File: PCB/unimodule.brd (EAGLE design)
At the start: 103 x 74.2 mm, 150 parts, among them IC1 TTGO_DISP, IC2 DS18D20, IC3 FAN3111E, IC4 FAN3111E, IC5 FAN3111E, K1 XY2500(5.0)-4PV, K100 G5LE-1-E 5VDC OMRON, K101 XY2500(5.0)-4PV, K102 JST-B02B-JWPF-SK-R, K103 JST-B04B-JWPF-SK-R, K104 JST-B08B-JWPF-SK-R, K105 JST-B03B-JWPF-SK-R, U1 MAX3485, U2 LMR62014XMFE/NOPB0

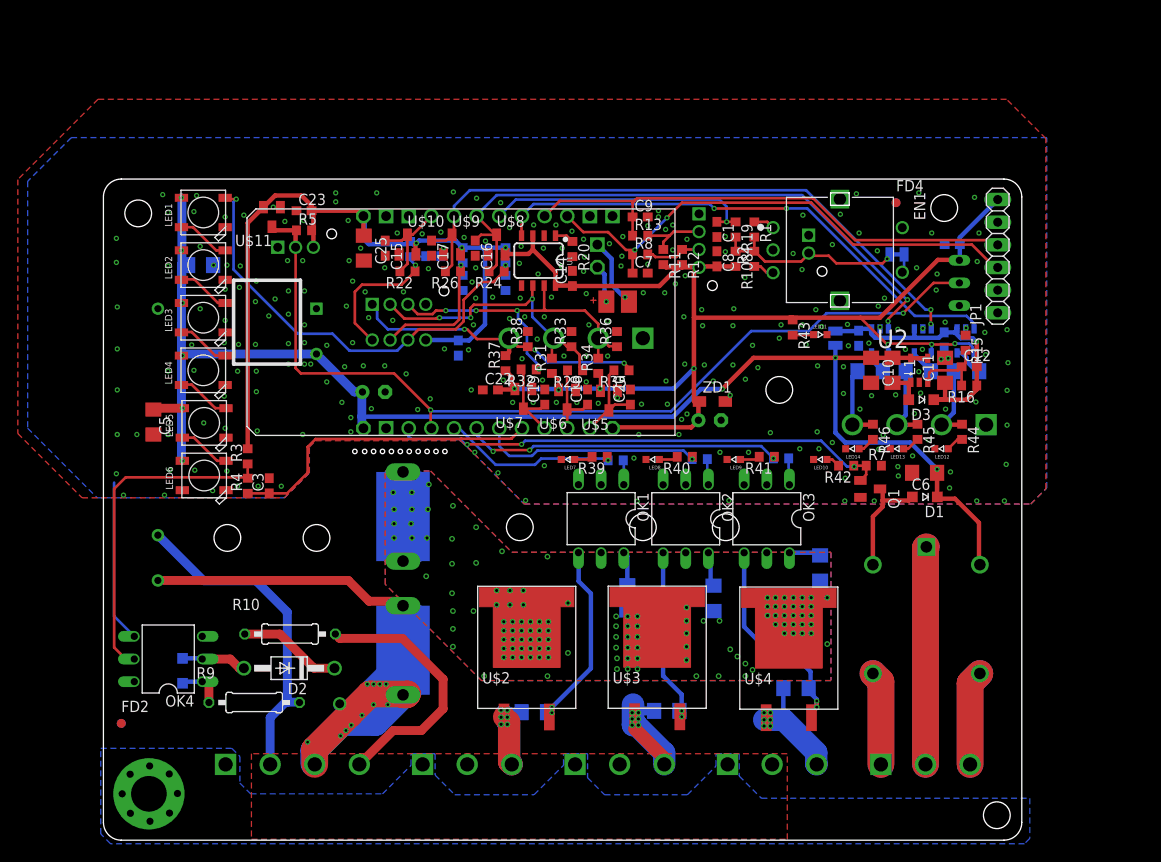
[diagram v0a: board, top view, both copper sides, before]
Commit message: silk screen organize
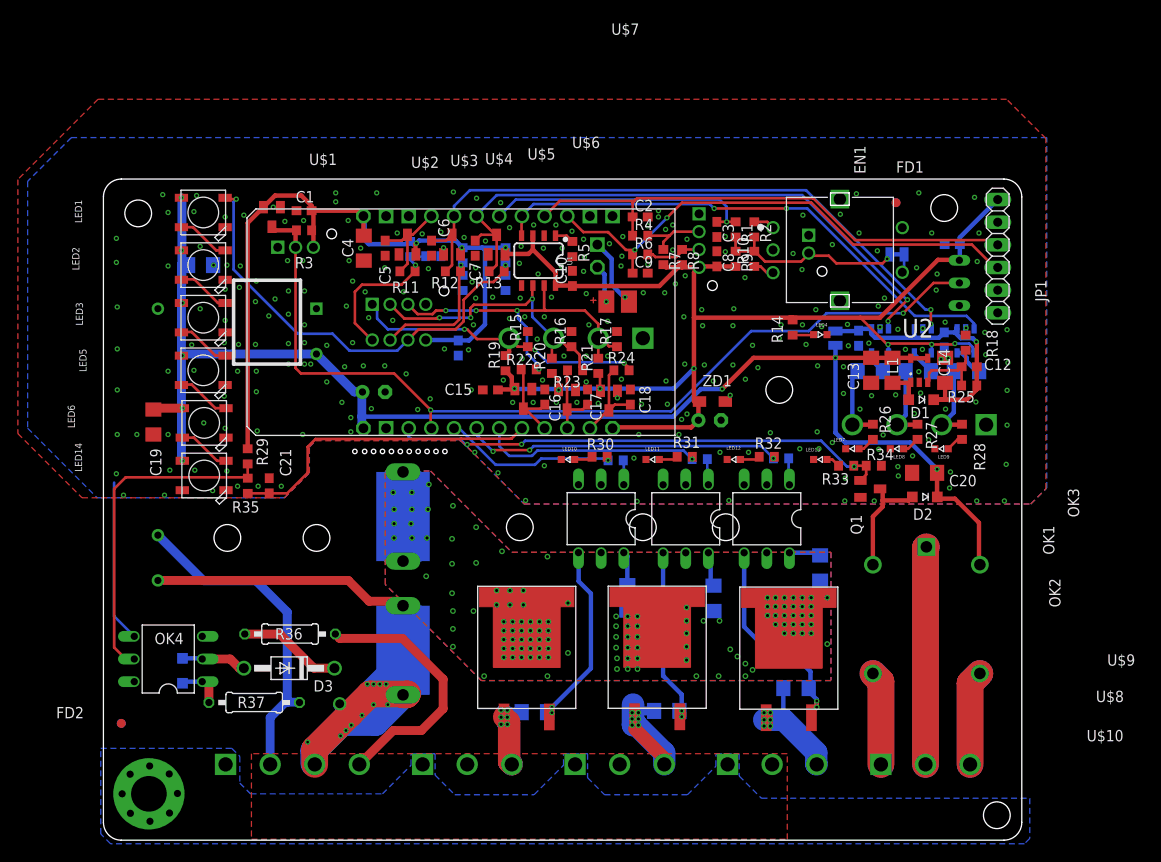
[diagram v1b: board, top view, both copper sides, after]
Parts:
- removed C22, C23: 100n, rcl:C0603
- removed C25: 22uF, rcl:C1206
- removed C26: DISP_BATSMD, TTGO_LCD_DISP:BAT_SMD
- removed FD3, FD4: (no value), siliXcon-pads:1-2MM-FIDUCIAL
- removed K1: XY2500(5.0)-4PV, siliXcon-connectors:XY2500V-B_4P
- removed R38: 10k, rcl:R0603
- removed R39, R40, R41, R42, R43: 220R, rcl:R0603
- removed R44, R45, R46: 1k, rcl:R0603
- removed SJ1: (no value), siliXcon-pads:SMD-JUMPER
- removed U$11: BAT54SFILM, siliXcon-semiconductors:PG-SOT23
- added C102, C103, C106: 100n, rcl:C0603
- added C105: 22uF, rcl:C1206
- added FD100, FD101: (no value), siliXcon-pads:1-2MM-FIDUCIAL
- added K106: JST-B03B-JWPF-SK-R, siliXcon-connectors:JST-B03B-JWPF-SK-R
- added R109, R110, R111: 1k, rcl:R1206
- added R112, R113, R114, R115, R116, R117: 10k, rcl:R0603
- added SJ101: (no value), siliXcon-pads:SMD-JUMPER-TIE
- added U$105: IRM-03-05, siliXcon-modules:IRM-03
- C1: value (none) -> 100n
- C10, C5, C6: value 22uF -> 100n; device rcl:C1206 -> rcl:C0603
- C11: value 22uF -> DISP_BATSMD; device rcl:C1206 -> TTGO_LCD_DISP:BAT_SMD
- C13, C14, C19, C20, C4: value 100n -> 22uF; device rcl:C0603 -> rcl:C1206
- C2: value 22uF -> !DNP 100n; device rcl:C1206 -> rcl:C0603
- C3: value 100n -> (none)
- C7: value !DNP 100n -> 100n
- D1: value (none) -> PMEG4005AEA
- D2: value 1N4004 -> (none); device diode:DO41-10 -> siliXcon-semiconductors:SOD123F
- D3: value PMEG4005AEA -> 1N4004; device siliXcon-semiconductors:SOD123F -> diode:DO41-10
- K102: value JST-B02B-JWPF-SK-R -> XY2500(5.0)-4PV; device siliXcon-connectors:JST-B02B-JWPF-SK-R -> siliXcon-connectors:XY2500V-B_4P
- K103: value JST-B04B-JWPF-SK-R -> JST-B08B-JWPF-SK-R; device siliXcon-connectors:JST-B04B-JWPF-SK-R -> siliXcon-connectors:JST-B08B-JWPF-SK-R
- K104: value JST-B08B-JWPF-SK-R -> JST-B04B-JWPF-SK-R; device siliXcon-connectors:JST-B08B-JWPF-SK-R -> siliXcon-connectors:JST-B04B-JWPF-SK-R
- K105: value JST-B03B-JWPF-SK-R -> JST-B02B-JWPF-SK-R; device siliXcon-connectors:JST-B03B-JWPF-SK-R -> siliXcon-connectors:JST-B02B-JWPF-SK-R
- LED14: value (none) -> WS2812B5050; device siliXcon-semiconductors:LED-0603 -> adafruit:WS2812B
- LED4: value WS2812B5050 -> (none); device adafruit:WS2812B -> siliXcon-semiconductors:LED-0603
- R10, R9: value 30k -> (none); device rcl:0207/10 -> rcl:R0603
- R105: value 220R -> 380R; device rcl:R0603 -> rcl:R1206
- R108: value (none) -> 220R
- R11, R12, R5: value 4k7 -> 100R
- R14: value 1k -> 220R; device rcl:R1206 -> rcl:R0603
- R15: value 6k8 -> 10k
- R16: value 47k -> 10k
- R17: value 1k -> 10k; device rcl:R1206 -> rcl:R0603
- R18: value 1k -> 6k8; device rcl:R1206 -> rcl:R0603
- R19: value (none) -> 10k
- R20: value 100R -> 10k
- R23: value 10k -> 100R
- R25: value 10k -> 47k
- R26, R29: value 100R -> 1k
- R27, R28: value 10k -> 1k
- R3: value 1k -> 4k7
- R30, R31, R33: value 10k -> 220R
- R32: value 100R -> 220R
- R34: value 10k -> 100k
- R35: value 100R -> 100k
- R36, R37: value 10k -> 30k; device rcl:R0603 -> rcl:0207/10
- R4: value 100k -> 100R
- R6: value 380R -> 100R; device rcl:R1206 -> rcl:R0603
- R7: value 100k -> 4k7
- R8: value 100R -> 4k7
- SJ100: device siliXcon-pads:SMD-JUMPER-TIE -> siliXcon-pads:SMD-JUMPER
- U$1: value IRM-03-05 -> BAT54SFILM; device siliXcon-modules:IRM-03 -> siliXcon-semiconductors:PG-SOT23
- U$10, U$8, U$9: value BAT54SFILM -> BT139B-600E; device siliXcon-semiconductors:PG-SOT23 -> siliXcon-semiconductors:D2PACK
- U$2, U$3, U$4: value BT139B-600E -> BAT54SFILM; device siliXcon-semiconductors:D2PACK -> siliXcon-semiconductors:PG-SOT23
- moved FD1 104.7 mm to (89.1, 72.0), flipped to the top
- moved D3 77.0 mm to (21.0, 19.8)
- moved D2 73.8 mm to (92.3, 39.0)
- moved R9 73.4 mm to (71.1, 65.7), turned to 270 degrees
- moved LED14 72.8 mm to (11.5, 41.4), turned to 180 degrees
- moved LED4 69.3 mm to (80.6, 57.2), turned to 270 degrees
- moved R10 66.9 mm to (73.2, 65.7), turned to 90 degrees
- moved C4 66.0 mm to (29.4, 66.9), flipped to the top, turned to 270 degrees
- moved U$10 63.3 mm to (77.1, 20.6)
- moved C6 60.8 mm to (37.0, 66.9), turned to 270 degrees
- moved R28 59.4 mm to (96.5, 46.3), flipped to the top
- moved C3 57.8 mm to (69.0, 69.0), turned to 270 degrees
- moved U$4 57.1 mm to (44.3, 67.3)
- moved K105 55.2 mm to (80.8, 64.3), turned to 90 degrees
- moved R25 54.0 mm to (97.3, 51.5), flipped to the top, turned to 180 degrees
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- renumbered C24 to C104, C27 to C107, IC2 to IC103, IC3 to IC100, IC4 to IC101, IC5 to IC102
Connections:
- removed net N$27 (its old number): LED4.2-DOUT, LED5.4-DIN
- new net N$28: LED14.4-DIN, LED6.2-DOUT
- net +10V: now also C103.2, C14.1, D1.C, R25.1, SJ100.2; no longer C11.1, C13.2, D3.C, R16.1, SJ1.2
- net +3V3: now also C1.2, C10.1, C102.2, C106.1, C15.2, K103.8, K104.4, K106.3, R115.1, R116.1, R117.1, R14.1, R19.1, R20.1, R29.2, R7.2, R8.2, R9.2, U$1.2, U$2.2, U$3.2, U$4.2; no longer C14.1, C21.2, C22.2, C23.2, C25.1, K103.4, K104.8, K105.3, R108.2, R11.2, R12.2, R25.1, R28.1, R31.1, R34.1, R37.1, R43.1, R5.2, U$10.2, U$11.2, U$8.2, U$9.2
- net +5V: now also C105.1, C13.1, C19.1, C20.1, D2.C, LED14.1-VDD, SJ100.1, U$105.V+; no longer C10.1, C2.1, C5.1, C6.1, D1.C, LED4.1-VDD, SJ1.1, U$1.V+
- net A1: now also K102.P$4, K103.1, R15.1, R19.2, R24.1; no longer K1.P$4, K104.1, R35.1, R37.2, R38.1
- net A2: now also K102.P$3, K103.2, R16.1, R20.2, R23.1; no longer K1.P$3, K104.2, R29.1, R31.2, R33.1
- net A3: now also K102.P$2, K103.3, R17.1, R21.2, R22.1; no longer K1.P$2, K104.3, R32.1, R34.2, R36.1
- net A4: now also K103.5, R11.1, R114.1, R117.2; no longer K104.5, R21.2, R22.1, R23.1
- net A5: now also K103.6, R113.1, R116.2, R12.1; no longer K104.6, R26.1, R28.2, R30.1
- net A6: now also K103.7, R112.1, R115.2, R13.1; no longer K104.7, R24.1, R25.2, R27.1
- net AIN_1: now also C18.1, R24.2, U$7.3; no longer C20.1, R35.2, U$5.3
- net AIN_2: now also C17.1, R23.2; no longer C18.1, R29.2
- net AIN_3: now also C16.1, R22.2, U$5.3; no longer C19.1, R32.2, U$7.3
- net AIN_4: now also C5.1, R11.2, U$2.3; no longer C15.1, R22.2, U$10.3
- net AIN_5/DO_2: now also C6.1, R12.2, U$3.3; no longer C17.1, R26.2, U$9.3
- net AIN_6/DO_3: now also C7.1, R13.2, U$4.3; no longer C16.1, R24.2, U$8.3
- net BAT+: now also C11.BAT+; no longer C26.BAT+
- net BAT-: now also C11.BAT-; no longer C26.BAT-
- net DALAS_TEMP: now also K106.2, R3.1, U$1.3; no longer K105.2, R5.1, U$11.3
- net ENC: now also C3.1, R1.1; no longer C1.1, R19.1
- net ENC_2: now also K105.2, R10.2, R9.1, SJ101.2; no longer K102.2, R108.1, R19.2, SJ100.2
- net GND: now also C1.1, C102.1, C103.1, C105.2, C106.2, C13.2, C15.1, C21.2, K102.P$1, K103.4, K104.1, K106.1, LED14.3-GND, LED4.C, R112.2, R113.2, R114.2, R15.2, R16.2, R17.2, R18.1, R34.2, R5.2, U$1.1, U$105.V-, U$2.1, U$3.1, U$4.1; no longer C1.2, C11.2, C13.1, C15.2, C21.1, C22.1, C23.1, C25.2, K1.P$1, K102.1, K103.1, K104.4, LED14.C, LED4.3-GND, R15.1, R20.2, R23.2, R27.2, R30.2, R33.2, R36.2, R38.2, R7.2, U$1.V-, U$10.1, U$11.1, U$8.1, U$9.1
- net L_FUSED: now also R105.1, U$10.2, U$8.2, U$9.2; no longer R6.1, U$2.2, U$3.2, U$4.2
- net L_IN: now also U$105.AC/L; no longer U$1.AC/L
- net L_OUT_1: now also R100.2, U$9.1; no longer R102.2, U$2.1
- net L_OUT_2: now also U$8.1; no longer U$3.1
- net L_OUT_3: now also R102.2, U$10.1; no longer R100.2, U$4.1
- net N: now also R37.2, U$105.AC/N; no longer R9.2, U$1.AC/N
- net N$1: now also D3.A; no longer D2.A
- net N$10: now also R107.2; no longer R105.2
- net N$11: now also R104.2; no longer R6.2
- net N$12: now also R100.1, U$9.3; no longer R102.1, U$2.3
- net N$13: now also R106.2; no longer R107.2
- net N$14: now also R10.1; no longer R2.1
- net N$15: now also SJ101.1; no longer SJ100.1
- net N$16: now also LED10.A, R30.2; no longer LED7.A, R39.2
- net N$17: now also LED11.A, R31.2; no longer LED8.A, R40.2
- net N$18: now also LED12.A, R32.2; no longer LED9.A, R41.2
- net N$2: now also D3.C, R36.1; no longer D2.C, R10.1
- net N$20: now also D2.A; no longer D1.A
- net N$21: now also LED13.A, R33.2; no longer LED10.A, R42.2
- net N$22: now also LED4.A, R14.2; no longer LED11.A, R43.2
- net N$23: now also R110.1; no longer R17.1
- net N$24: now also D1.A; no longer D3.A
- net N$26: now also LED5.4-DIN; no longer LED4.4-DIN
- net N$29: now also LED9.A, R28.2; no longer LED12.A, R44.2
- net N$3: now also R2.1; no longer R1.1
- net N$30: now also LED8.A, R27.2; no longer LED13.A, R45.2
- net N$31: now also R109.1; no longer R14.1
- net N$32: now also LED7.A, R26.2; no longer LED14.A, R46.2
- net N$33: now also R111.1; no longer R18.1
- net N$34: now also R18.2, R25.2; no longer R15.2, R16.2
- net N$38: now also R5.1; no longer R20.1
- net N$4: now also R37.1; no longer R9.1
- net N$5: now also R105.2; no longer R103.2
- net N$6: now also R102.1, U$10.3; no longer R100.1, U$4.3
- net N$7: now also R103.2; no longer R104.2
- net N$8: now also R108.2; no longer R106.2
- net N$9: now also U$8.3; no longer U$3.3
- net OUT_1_SIG: now also R106.1, R30.1; no longer R107.1, R39.1
- net OUT_2_SIG: now also R107.1, R31.1; no longer R105.1, R40.1
- net OUT_3_SIG: now also R108.1, R32.1; no longer R106.1, R41.1
- net PWM_1: now also R109.2, R28.1; no longer R14.2, R44.1
- net PWM_2: now also R110.2, R27.1; no longer R17.2, R45.1
- net PWM_3: now also R111.2, R26.1; no longer R18.2, R46.1
- net RELAY_SIG: now also R33.1, R34.1; no longer R42.1, R7.1
- net SCL: now also C2.1, R4.1; no longer C9.1, R13.1
- net SCL_P: now also K104.2, R4.2, R7.1; no longer K103.2, R11.1, R13.2
- net SDA: now also C9.1, R6.1; no longer C7.1, R8.1
- net SDA_P: now also K104.3, R6.2, R8.1; no longer K103.3, R12.1, R8.2
- net SENS_IN: now also R36.2; no longer R10.2
- net ZC: now also R29.1, R35.2; no longer R3.1, R4.2
- net ZC_SIG: now also C21.1, R35.1; no longer C3.1, R4.1
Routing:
- net N$27 (its old number): track 6.12 -> 0.00 mm
- net N$28: track 0.00 -> 5.98 mm
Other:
- board text added: "2020"
- board text added: "Matous Cmelik"
- board text removed: "Matous Cmelik 2020"
